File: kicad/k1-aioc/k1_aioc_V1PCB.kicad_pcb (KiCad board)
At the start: 2 copper layers, 63 parts, among them J1 Conn_01x07_Male, J2 12401832E402A, J3 SIP 200, J4 SIP 200, T1 Transformer_Audio_CTP_CTS, T2 Transformer_Audio_CTP_CTS, U1 MIC5330-SSYML, U2 STM32F373CBTx(OLD), U3 4N25, U4 4N25, Y1 8MHz/20pF

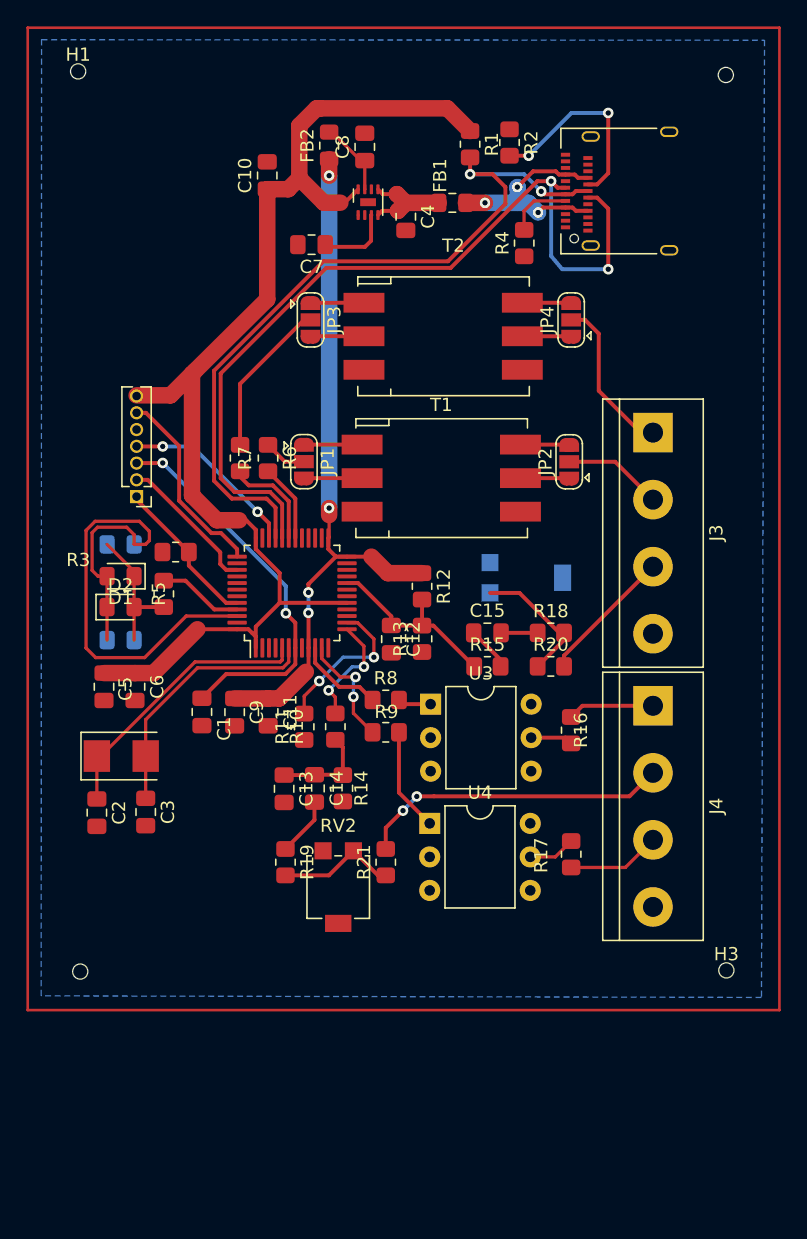
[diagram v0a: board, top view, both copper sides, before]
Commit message: Updating Kicad files for review
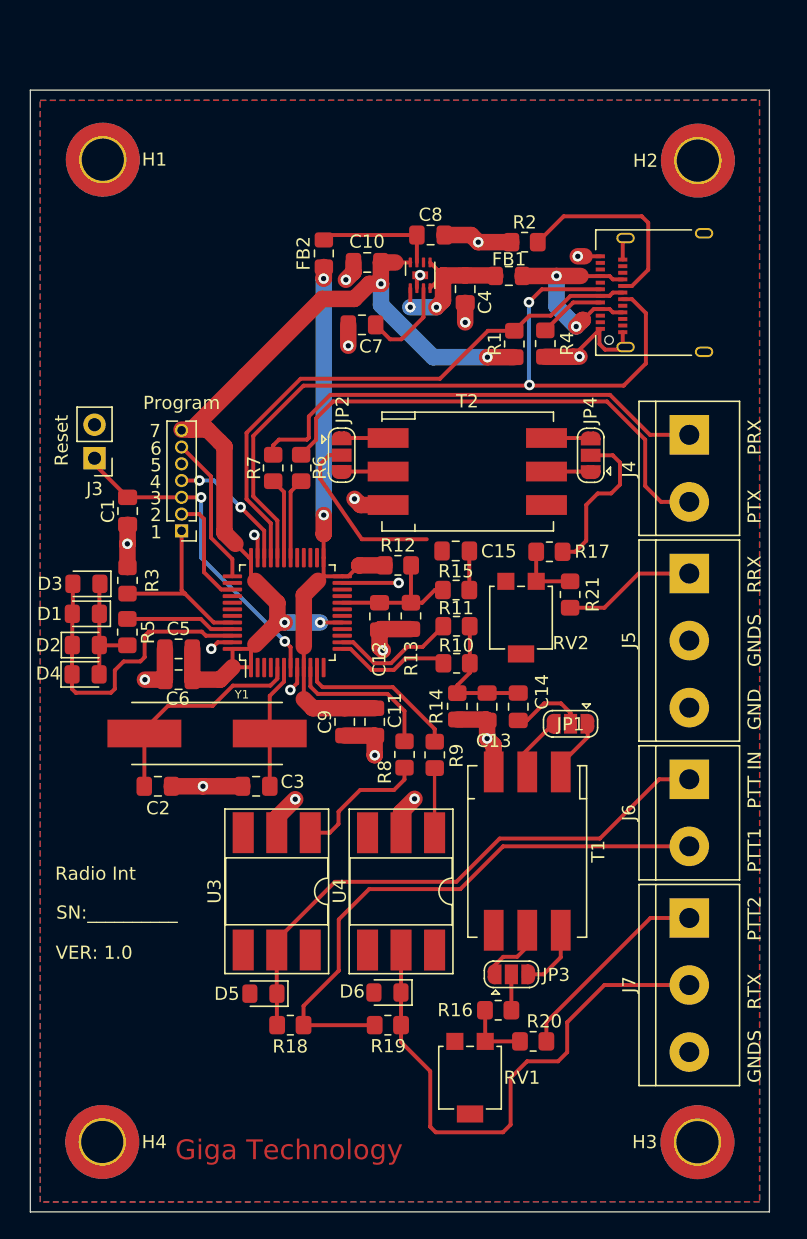
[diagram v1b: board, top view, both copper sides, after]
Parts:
- removed the R16 at (149.4, 105.7)
- removed the R17 at (149.4, 115.1)
- added D5: 1N4001, Diode_SMD:D_0805_2012Metric_Pad1.15x1.40mm_HandSolder, F.Cu at (126.1, 125.7)
- added D6: 1N4001, Diode_SMD:D_0805_2012Metric_Pad1.15x1.40mm_HandSolder, F.Cu at (135.5, 125.6)
- added J5: SIP 200, TerminalBlock:TerminalBlock_bornier-3_P5.08mm, F.Cu at (158.3, 93.8)
- added J6: SIP 200, TerminalBlock:TerminalBlock_bornier-2_P5.08mm, F.Cu at (158.3, 109.4)
- added J7: SIP 200, TerminalBlock:TerminalBlock_bornier-3_P5.08mm, F.Cu at (158.3, 119.9)
- added R18: 1K2, Resistor_SMD:R_0805_2012Metric_Pad1.20x1.40mm_HandSolder, F.Cu at (128.1, 128.1)
- added R19: 1K2, Resistor_SMD:R_0805_2012Metric_Pad1.20x1.40mm_HandSolder, F.Cu at (135.5, 128.1)
- D3, D4: moved to F.Cu
- H1, H2, H3, H4: footprint AIOC:TOOLING-HOLE -> MountingHole:MountingHole_3.2mm_M3_DIN965_Pad_TopBottom
- J3: value SIP 200 -> conn_01X02; footprint TerminalBlock:TerminalBlock_bornier-4_P5.08mm -> Connector_PinHeader_2.54mm:PinHeader_1x02_P2.54mm_Vertical
- J4: footprint TerminalBlock:TerminalBlock_bornier-4_P5.08mm -> TerminalBlock:TerminalBlock_bornier-2_P5.08mm
- RV2: renamed from RV1; moved to F.Cu
- U3, U4: footprint Package_DIP:DIP-6_W7.62mm -> Package_DIP:DIP-6_W8.89mm_SMDSocket_LongPads
- Y1: footprint AIOC:Crystal_SMD_5032-2Pin_5.0x3.2mm -> AIOC:Crystal_8MHz_SMD_11.40mm
- moved J3 42.4 mm to (113.3, 85.1), turned to 180 degrees
- moved JP3 39.1 mm to (144.9, 124.2), turned to 0 degrees
- moved T1 29.0 mm to (146.1, 114.9), turned to -90 degrees
- moved JP1 28.3 mm to (149.4, 105.2), turned to 180 degrees
- moved J4 20.7 mm to (158.3, 83.3)
- moved R16 19.6 mm to (143.9, 126.9), turned to 180 degrees
- moved U3 18.4 mm to (127.1, 117.9), turned to -90 degrees
- moved R20 17.6 mm to (146.5, 129.3), turned to 0 degrees
- moved RV1 17.6 mm to (141.7, 132.0)
- moved C14 16.6 mm to (145.4, 103.9)
- moved C13 16.6 mm to (143.0, 103.9)
- moved C1 16.2 mm to (115.8, 89.1)
- moved R1 15.5 mm to (145.1, 76.4), turned to 90 degrees
- moved R11 13.8 mm to (140.7, 97.8), turned to 180 degrees
- moved H3 13.2 mm to (159.0, 136.9)
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- renumbered JP3 to JP2, JP2 to JP3, R19 to R16, R18 to R17, R21 to R20, R20 to R21, RV2 to RV1
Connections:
- J3 pad 1: Net-(JP4-Pad2) -> /NRST
- J3 pad 2: /RADIO-RX-PTT1 -> GND
- J4 pad 1: /RADIO-VP-PTT2 -> Net-(J4-Pad1)
- JP1 pad 2: Net-(JP1-Pad2) -> Net-(C14-Pad2)
- JP2 pad 2: Net-(JP3-Pad2) -> Net-(C15-Pad2)
- JP3 pad 2: /RADIO-RX-PTT1 -> Net-(JP3-Pad2)
- R16 pad 1: Net-(C14-Pad2) -> Net-(JP3-Pad2)
- R17 pad 1: Net-(C15-Pad2) -> Net-(JP4-Pad2)
- R20 pad 2: Net-(J4-Pad2) -> Net-(J7-Pad1)
- R21 pad 2: Net-(J3-Pad3) -> Net-(J5-Pad1)
- R6 pad 1: Net-(JP1-Pad2) -> Net-(J4-Pad2)
- R7 pad 1: Net-(JP3-Pad2) -> Net-(J4-Pad1)
- RV1 pad 2: GND -> GNDS
- RV1 pad 3: GND -> GNDS
- RV2 pad 2: GND -> GNDS
- RV2 pad 3: GND -> GNDS
- T1 pad 4: GND -> GNDS
- T2 pad 4: GND -> GNDS
- U3 pad 5: Net-(R16-Pad2) -> /RADIO-VP-PTT2
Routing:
- net GND: track 0.00 -> 69.8 mm, vias 0 -> 20
- net Net-(J6-Pad2): track 0.00 -> 43.4 mm
- net Net-(D6-Pad1): track 3.60 -> 42.1 mm
- net /RADIO-VP-PTT2: track 6.55 -> 42.8 mm
- net Net-(J4-Pad1): track 0.00 -> 36.0 mm
- net Net-(D1-Pad2): track 42.7 -> 24.1 mm
- net +3V3: track 91.6 -> 74.1 mm, vias 0 -> 4
- net /USB-DP: track 58.8 -> 43.1 mm, vias 2 -> 0
- net Net-(J7-Pad1): track 0.00 -> 15.6 mm
- net /RADIO-RX-PTT1: track 14.6 -> 0.00 mm
- net Net-(J4-Pad2): track 23.6 -> 37.2 mm, vias 2 -> 0
- net Net-(C15-Pad2): track 2.77 -> 13.5 mm
- net Net-(J3-Pad3): track 10.3 -> 0.00 mm
- net /OSCOUT: track 19.7 -> 9.45 mm
- net Net-(J5-Pad1): track 0.00 -> 10.1 mm
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- added copper zone on F.Cu, net GNDS
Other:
- board outline added: 56 x 85 mm
- board text added: "1"
- board text added: "2"
- board text added: "3"
- board text added: "4"
- board text added: "5"
- board text added: "6"
- board text added: "7"
- board text added: "GND"
- board text added: "GNDS"
- board text added: "Giga Technology"
- board text added: "PRX"
- board text added: "PTT IN"
- board text added: "PTT1"
- board text added: "PTT2"
- board text added: "PTX"
- board text added: "Program"
- board text added: "RRX"
- board text added: "RTX"
- board text added: "Radio Int"
- board text added: "Reset"
- board text added: "SN:__________"
- board text added: "VER: 1.0"
